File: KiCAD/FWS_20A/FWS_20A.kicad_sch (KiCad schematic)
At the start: 74 parts, among them J1 pwr, J2 Conn_01x02_Pin, J3 Conn_01x09_Socket, J4 Conn_01x02_Pin, J5 sense, Q1 DMN32D2LDF, Q6 DMN32D2LDF, SW2 SW_Push, U1 XMSM0L1306SRGER, U11 FCX495, U12 ADS1015IDGS, U2 FDMS8333L, U3 FDMS8333L, U4 LM5109BSD, U5 LM5109BSD, U6 L78L33_SO8, U7 FDMS8333L, U8 FDMS8333L

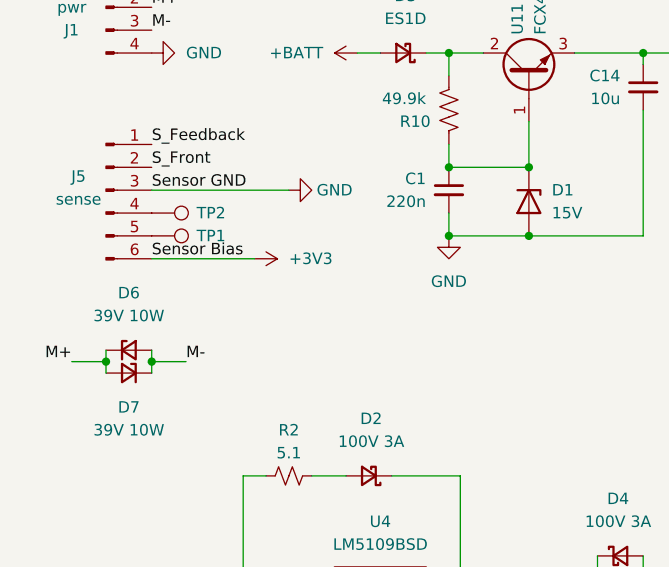
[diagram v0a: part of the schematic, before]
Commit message: asd
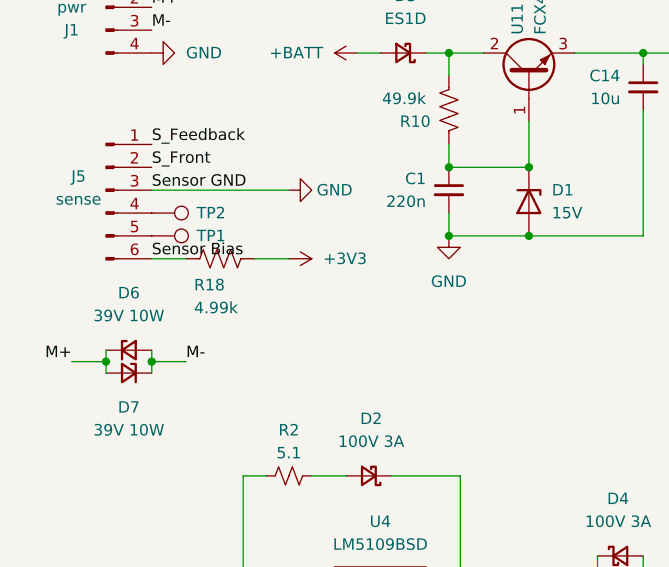
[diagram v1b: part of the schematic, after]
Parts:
- added R18: 4.99k, Resistor_SMD:R_1206_3216Metric_Pad1.30x1.75mm_HandSolder, symbol Device:R_US
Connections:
- net +3V3: now also R18.1; no longer J5.6 (Pin_6)
- new net Sensor Bias: J5.6 (Pin_6), R18.2
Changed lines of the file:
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@@
 	(wire
 		(pts
+			(xy 40.64 52.07) (xy 44.45 52.07)
+		)
+		(stroke
+			(width 0)
+			(type default)
+		)
+	)
+	(wire
+		(pts
 			(xy 46.99 76.2) (xy 50.8 76.2)
 		)
@@
 	(wire
 		(pts
-			(xy 29.21 52.07) (xy 40.64 52.07)
+			(xy 29.21 52.07) (xy 33.02 52.07)
 		)
 		(stroke
@@
 	)
 	(symbol
+		(lib_id "Device:R_US")
+		(at 36.83 52.07 270)
+		(unit 1)
+		(exclude_from_sim no)
+		(in_bom yes)
+		(on_board yes)
+		(dnp no)
+		(property "Reference" "R18"
+			(at 33.909 54.991 90)
+			(effects
+				(font
+					(size 1.27 1.27)
+				)
+				(justify left)
+			)
+		)
+		(property "Value" "4.99k"
+			(at 33.909 57.531 90)
+			(effects
+				(font
+					(size 1.27 1.27)
+				)
+				(justify left)
+			)
+		)
+		(property "Footprint" "Resistor_SMD:R_1206_3216Metric_Pad1.30x1.75mm_HandSolder"
+			(at 36.576 53.086 90)
+			(effects
+				(font
+					(size 1.27 1.27)
+				)
+				(hide yes)
+			)
+		)
+		(property "Datasheet" ""
+			(at 36.83 52.07 0)
+			(effects
+				(font
+					(size 1.27 1.27)
+				)
+				(hide yes)
+			)
+		)
+		(property "Description" "Resistor, US symbol"
+			(at 36.83 52.07 0)
+			(effects
+				(font
+					(size 1.27 1.27)
+				)
+				(hide yes)
+			)
+		)
+		(property "Sim.Device" ""
+			(at 36.83 52.07 90)
+			(effects
+				(font
+					(size 1.27 1.27)
+				)
+				(hide yes)
+			)
+		)
+		(property "Sim.Type" ""
+			(at 36.83 52.07 90)
+			(effects
+				(font
+					(size 1.27 1.27)
+				)
+				(hide yes)
+			)
+		)
+		(property "mouser" "https://www.mouser.com/ProductDetail/SEI-Stackpole/RNCP1206FTD4K99?qs=sGAEpiMZZMvdGkrng054tyMPH50YnZ95yR%2FF2bQQIaAb5UdPiGbTtQ%3D%3D"
+			(at 36.83 52.07 0)
+			(effects
+				(font
+					(size 1.27 1.27)
+				)
+				(hide yes)
+			)
+		)
+		(property "specs" "4.99kOhm, 200V, 500mW, 1%, 100PPM, -55C, +155C"
+			(at 36.83 52.07 0)
+			(effects
+				(font
+					(size 1.27 1.27)
+				)
+				(hide yes)
+			)
+		)
+		(property "unit x10" "0.017"
+			(at 36.83 52.07 0)
+			(effects
+				(font
+					(size 1.27 1.27)
+				)
+				(hide yes)
+			)
+		)
+		(pin "1"
+		)
+		(pin "2"
+		)
+		(instances
+			(project "FWS_20A"
+				(path "/bd07da4b-c018-42fa-9039-1b3b7c5adf19"
+					(reference "R18")
+					(unit 1)
+				)
+			)
+		)
+	)
+	(symbol
 		(lib_id "Regulator_Linear:L78L33_SO8")
 		(at 119.38 29.21 0)
@@
 	(symbol
 		(lib_id "power:+3V3")
-		(at 40.64 52.07 270)
+		(at 44.45 52.07 270)
 		(unit 1)
 		(exclude_from_sim no)
@@
 		(fields_autoplaced yes)
 		(property "Reference" "#PWR018"
-			(at 36.83 52.07 0)
+			(at 40.64 52.07 0)
 			(effects
 				(font
@@
 		)
 		(property "Value" "+3V3"
-			(at 44.45 52.0699 90)
+			(at 48.26 52.0699 90)
 			(effects
 				(font
@@
 		)
 		(property "Footprint" ""
-			(at 40.64 52.07 0)
+			(at 44.45 52.07 0)
 			(effects
 				(font
@@
 		)
 		(property "Datasheet" ""
-			(at 40.64 52.07 0)
+			(at 44.45 52.07 0)
 			(effects
 				(font
@@
 		)
 		(property "Description" "Power symbol creates a global label with name \"+3V3\""
-			(at 40.64 52.07 0)
+			(at 44.45 52.07 0)
 			(effects
 				(font
